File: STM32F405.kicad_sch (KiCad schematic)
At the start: 25 parts, among them SW1 SW_MEC_5G, U6 STM32F405RGTx, Y1 25MHz, Y2 Crystal

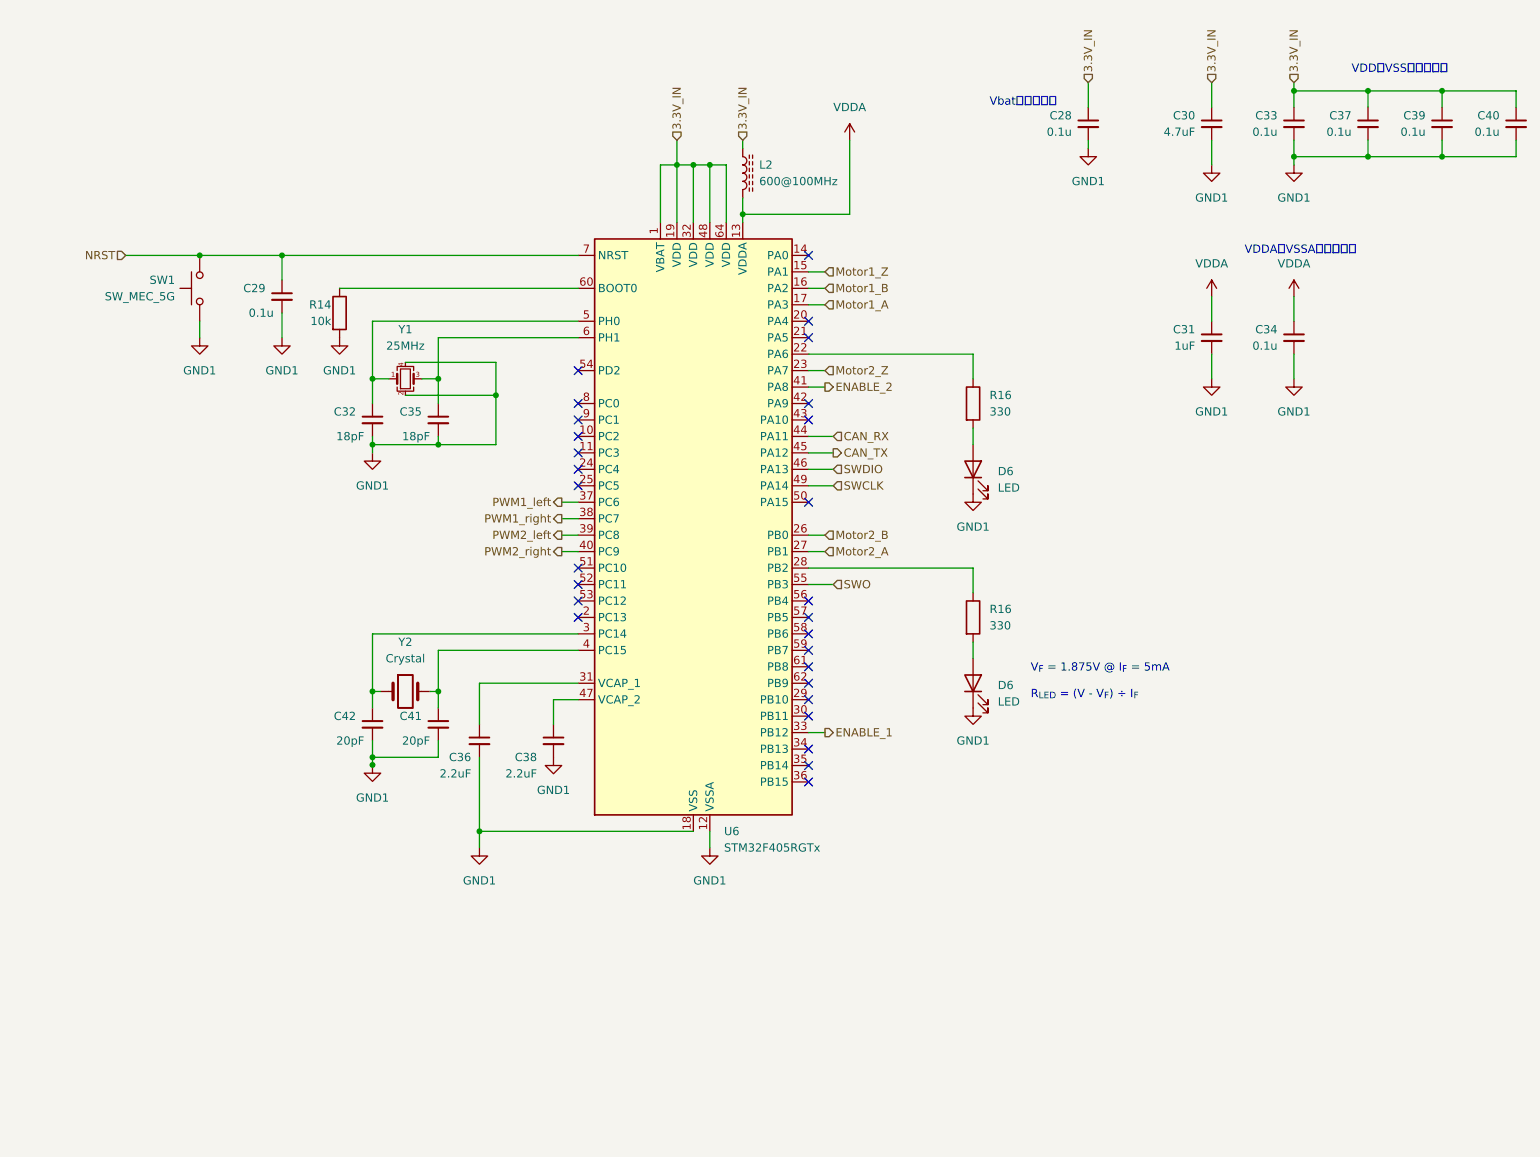
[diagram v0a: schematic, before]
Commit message: release prot.1 v0.1.0
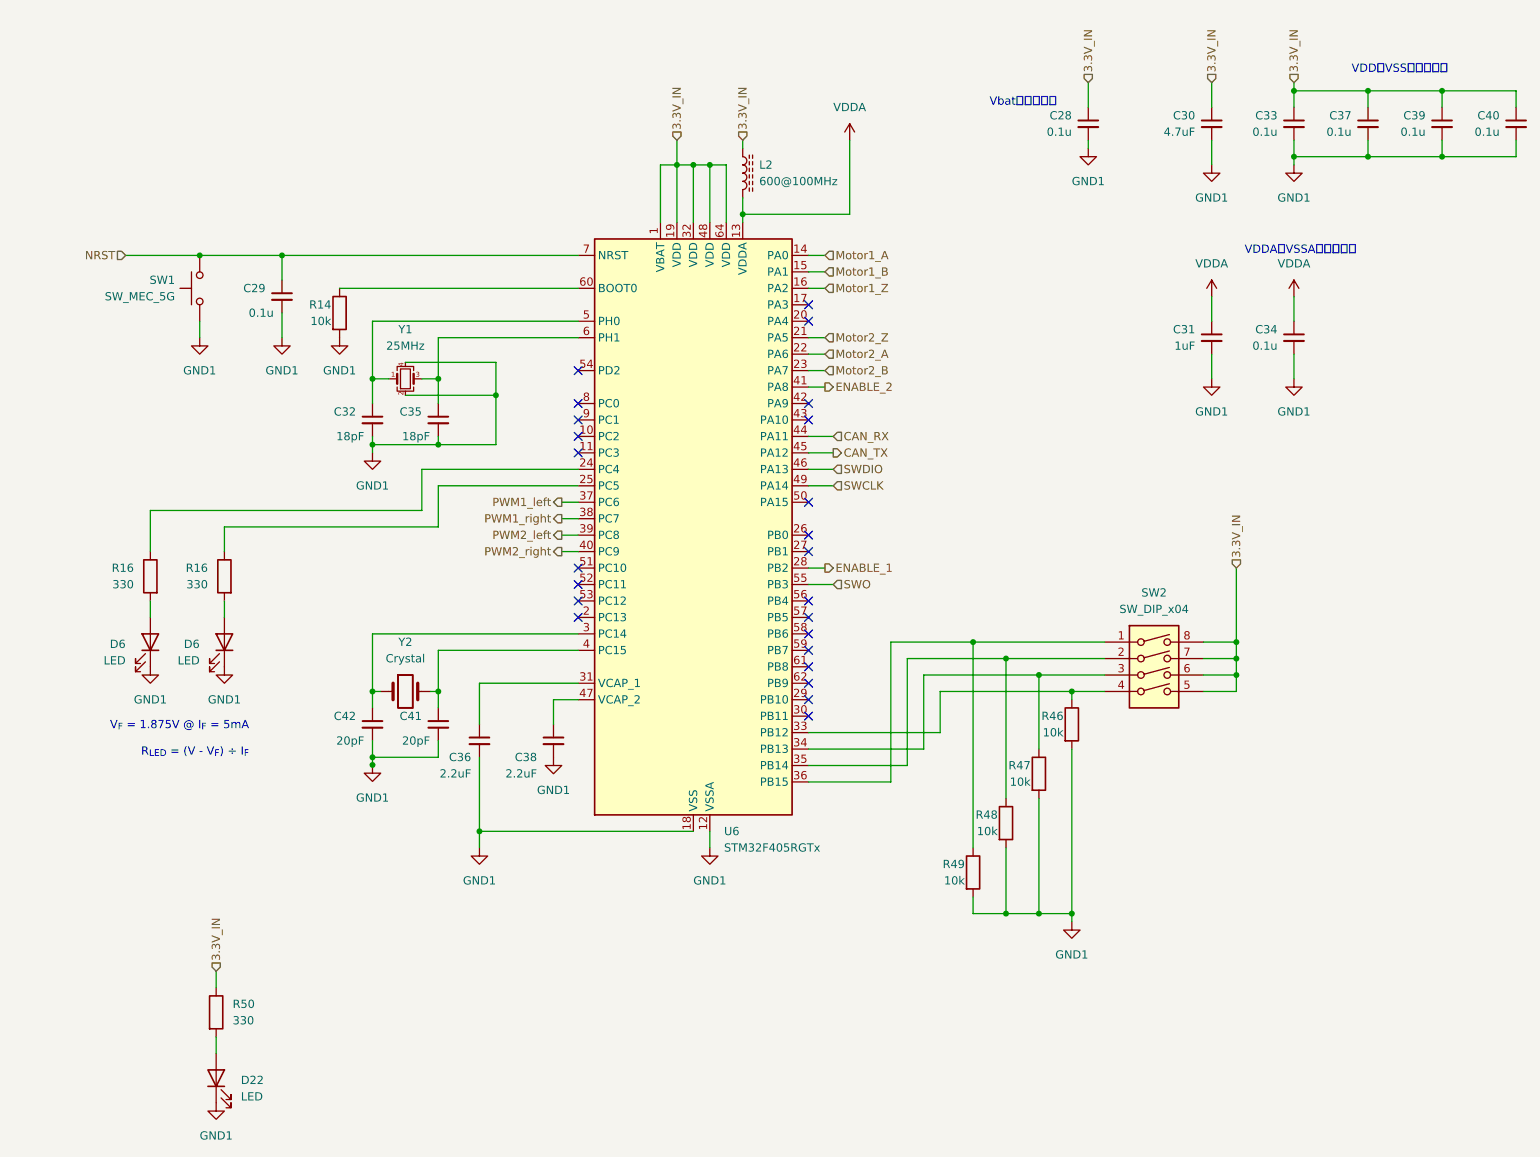
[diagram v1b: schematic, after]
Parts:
- added D22: LED, LED_SMD:LED_0603_1608Metric_Pad1.05x0.95mm_HandSolder, symbol Device:LED
- added R46, R47, R48, R49: 10k, Resistor_SMD:R_0402_1005Metric_Pad0.72x0.64mm_HandSolder, symbol Device:R
- added R50: 330, Resistor_SMD:R_0603_1608Metric_Pad0.98x0.95mm_HandSolder, symbol Device:R
- added SW2: SW_DIP_x04, Button_Switch_SMD:SW_DIP_SPSTx04_Slide_Copal_CHS-04B_W7.62mm_P1.27mm, symbol Switch:SW_DIP_x04
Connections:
- net 3.3V_IN: now also R50.1, SW2.5, SW2.6, SW2.7, SW2.8
- net ENABLE_1: now also U6.28 (PB2); no longer U6.33 (PB12)
- net GND1: now also D22.1 (K), R46.2, R47.2, R48.2, R49.2
- net Motor1_A: now also U6.14 (PA0); no longer U6.17 (PA3)
- net Motor1_B: now also U6.15 (PA1); no longer U6.16 (PA2)
- net Motor1_Z: now also U6.16 (PA2); no longer U6.15 (PA1)
- net Motor2_A: now also U6.22 (PA6); no longer U6.27 (PB1)
- net Motor2_B: now also U6.23 (PA7); no longer U6.26 (PB0)
- net Motor2_Z: now also U6.21 (PA5); no longer U6.23 (PA7)
- net at R16.1: now also U6.24 (PC4); no longer U6.22 (PA6)
- net at U6.25 (PC5): now also R16.1
- net at U6.34 (PB13): now also R47.1, SW2.3
- net at U6.35 (PB14): now also R48.1, SW2.2
- net at U6.36 (PB15): now also R49.1, SW2.1
- new net: D22.2 (A), R50.2
- new net: R46.1, SW2.4, U6.33 (PB12)
- no-connect marks 28 -> 24
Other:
- moved on the sheet: D6, R16

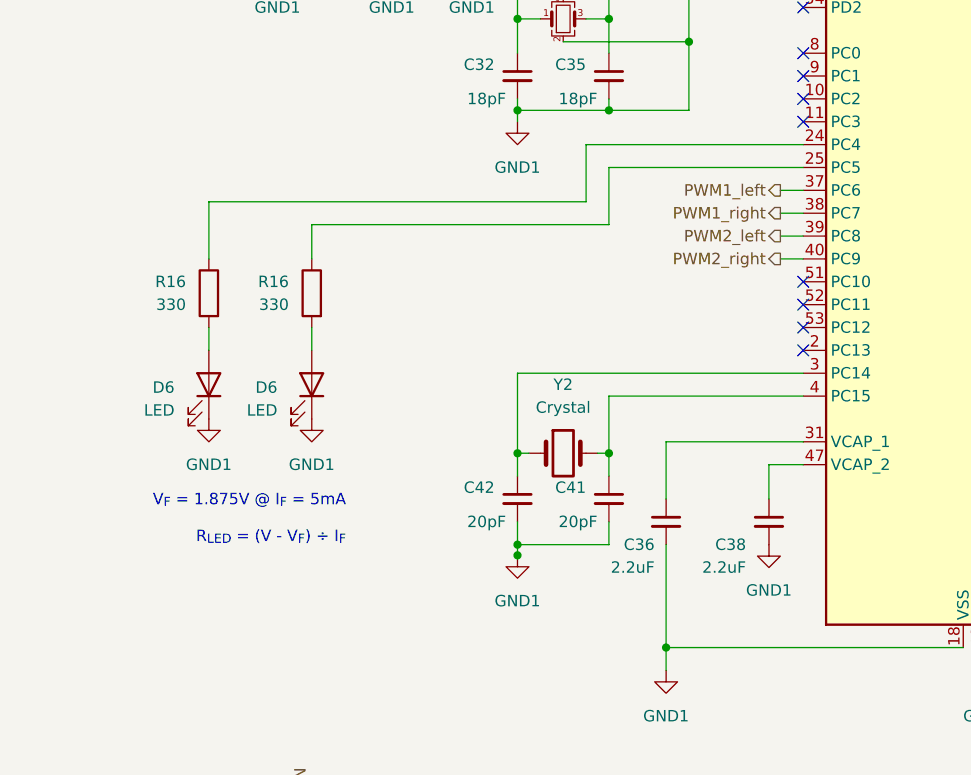
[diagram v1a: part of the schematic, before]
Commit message: add branch v0.2.0
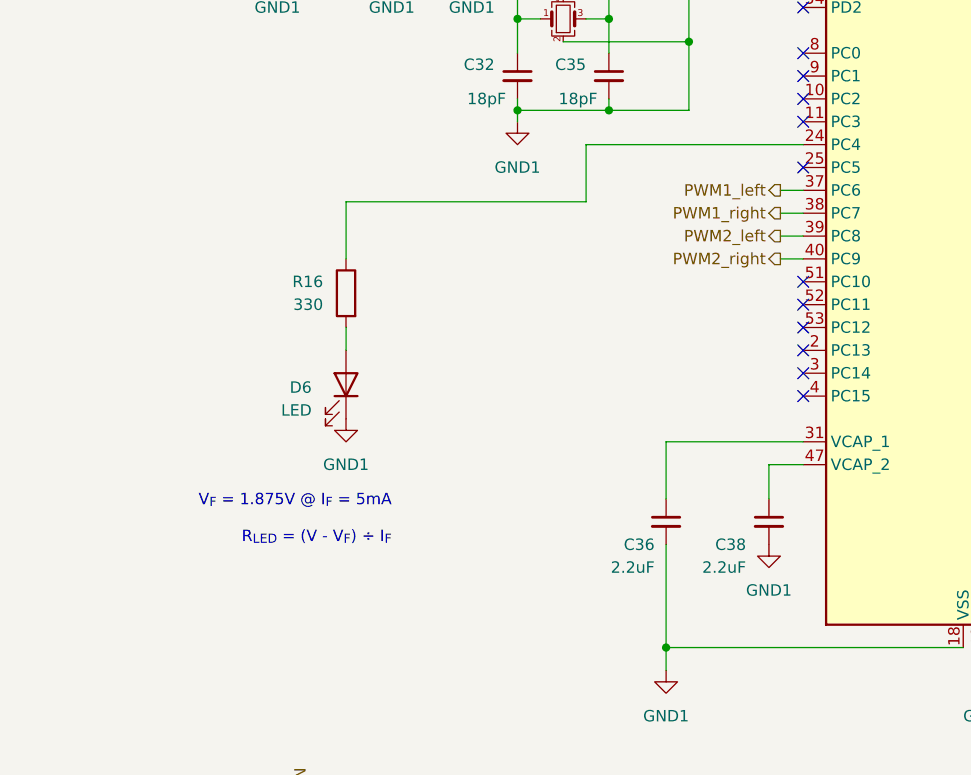
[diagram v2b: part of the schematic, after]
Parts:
- removed C41, C42: 20pF, Capacitor_SMD:C_0402_1005Metric, symbol Device:C_Small
- removed D6: LED, LED_SMD:LED_0805_2012Metric, symbol Device:LED
- removed R16: 330, Resistor_SMD:R_0603_1608Metric_Pad0.98x0.95mm_HandSolder, symbol Device:R
- removed Y2: Crystal, Crystal:Crystal_SMD_3215-2Pin_3.2x1.5mm, symbol Device:Crystal
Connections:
- no-connect marks 24 -> 27
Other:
- moved on the sheet: D6, R16
